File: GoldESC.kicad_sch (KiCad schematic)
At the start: 42 parts, among them J30 CanOut, J4 GND, J5 DB15_Female_HighDensity, J81 Conn_02x07_Counter_Clockwise, U2 FD8288T (DRV8300), U30 MCP2551-I-SN, U31 CPDT-12V, U80 STM32F103CBTx, U81 ABM3B-8.000MHZ

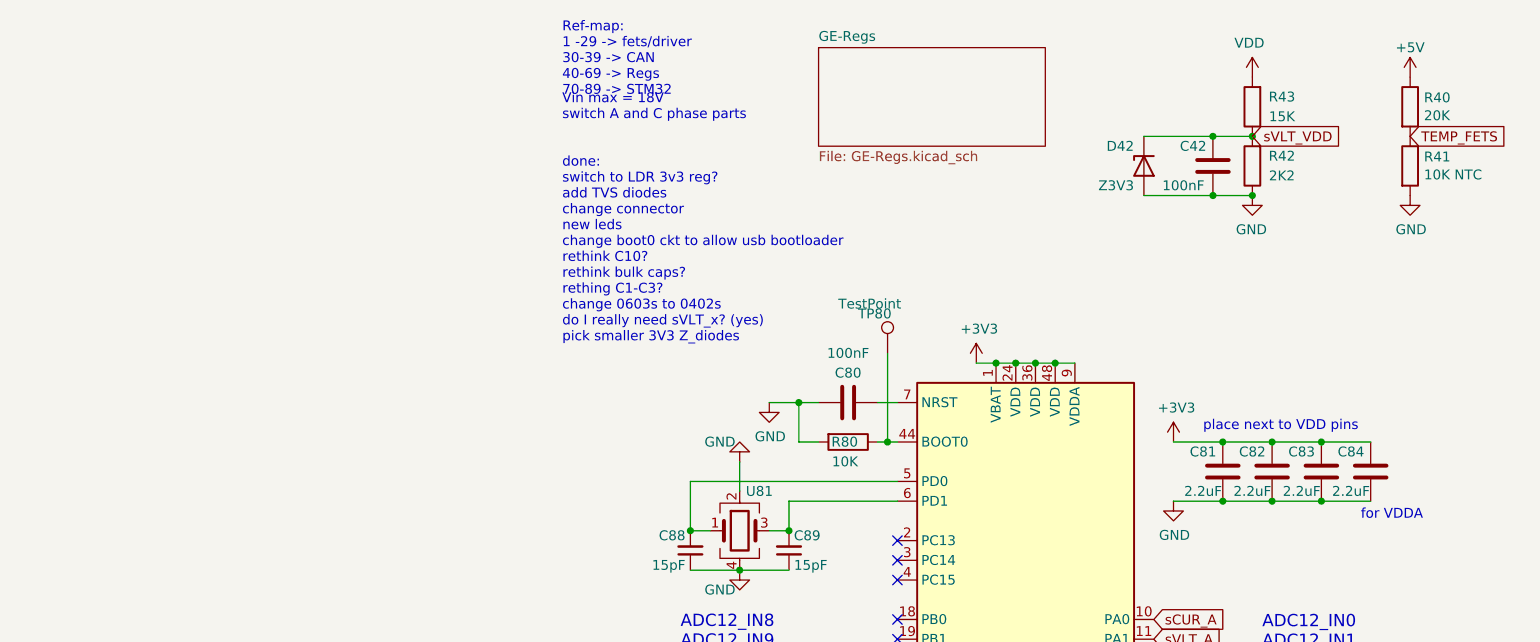
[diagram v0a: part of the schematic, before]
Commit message: updated gitignore
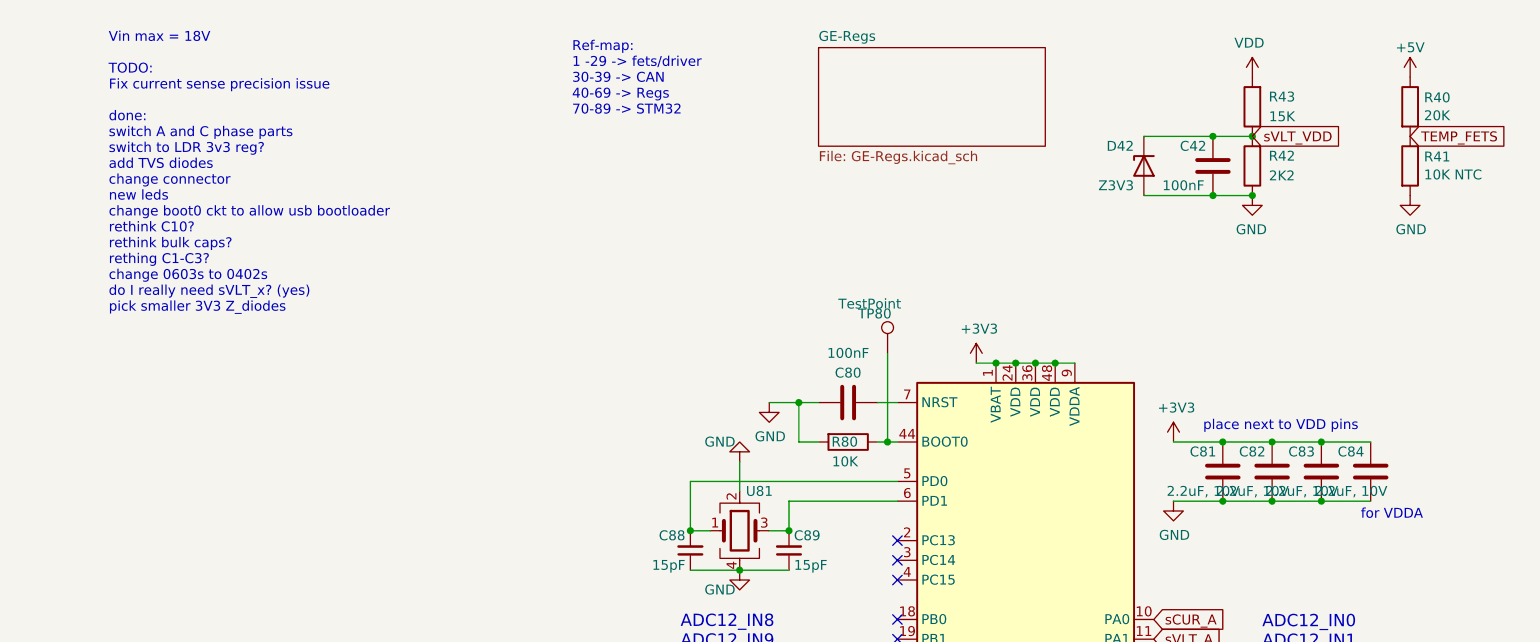
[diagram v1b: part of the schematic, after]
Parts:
- C81, C82, C83, C84: value 2.2uF -> 2.2uF, 10V; LCSC C12530 -> C77002
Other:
- note added: "Vin max = 18V TODO: Fix current sense precision issue done: switch A and C phase parts switch to LDR 3v3 reg? add TVS diodes change connector new leds change boot0 ckt to allow usb bootloader rethink C10? rethink bulk caps? rething C1-C3? change 0603s to 0402s do I really need sVLT_x? (yes) pick smaller 3V3 Z_diodes"
- note removed: "Vin max = 18V switch A and C phase parts done: switch to LDR 3v3 reg? add TVS diodes change connector new leds change boot0 ckt to allow usb bootloader rethink C10? rethink bulk caps? rething C1-C3? change 0603s to 0402s do I really need sVLT_x? (yes) pick smaller 3V3 Z_diodes"
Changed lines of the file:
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@@
     (stroke (width 0) (type default) (color 0 0 0 0))
   )
-  (text "Vin max = 18V\nswitch A and C phase parts\n\n\ndone:\nswitch to LDR 3v3 reg?\nadd TVS diodes\nchange connector\nnew leds\nchange boot0 ckt to allow usb bootloader\nrethink C10?\nrethink bulk caps?\nrething C1-C3?\nchange 0603s to 0402s\ndo I really need sVLT_x? (yes)\npick smaller 3V3 Z_diodes"
-    (at 13.97 55.88 0)
+  (text "Vin max = 18V\n\nTODO:\nFix current sense precision issue\n\ndone:\nswitch A and C phase parts\nswitch to LDR 3v3 reg?\nadd TVS diodes\nchange connector\nnew leds\nchange boot0 ckt to allow usb bootloader\nrethink C10?\nrethink bulk caps?\nrething C1-C3?\nchange 0603s to 0402s\ndo I really need sVLT_x? (yes)\npick smaller 3V3 Z_diodes"
+    (at -44.45 52.07 0)
     (effects (font (size 1.27 1.27)) (justify left bottom))
   )
@@
   )
   (text "Ref-map:\n1 -29 -> fets/driver\n30-39 -> CAN\n40-69 -> Regs\n70-89 -> STM32"
-    (at 13.97 24.13 0)
+    (at 15.24 26.67 0)
     (effects (font (size 1.27 1.27)) (justify left bottom))
   )
@@
     (in_bom yes) (on_board yes)
     (property "Reference" "C83" (id 0) (at 109.22 69.85 0))
-    (property "Value" "2.2uF" (id 1) (at 109.22 74.93 0))
+    (property "Value" "2.2uF, 10V" (id 1) (at 109.22 74.93 0))
     (property "Footprint" "Capacitor_SMD:C_0402_1005Metric" (id 2) (at 112.7252 76.2 0)
       (effects (font (size 1.27 1.27)) hide)
     )
-    (property "Datasheet" "https://lcsc.com/product-detail/Multilayer-Ceramic-Capacitors-MLCC---SMD-SMT_Samsung-Electro-Mechanics-Samsung-Electro-Mechanics-CL05A225MQ5NSNC_C12530.html" (id 3) (at 111.76 72.39 0)
-      (effects (font (size 1.27 1.27)) hide)
-    )
-    (property "LCSC" "C12530" (id 4) (at 111.76 72.39 0)
+    (property "Datasheet" "https://lcsc.com/product-detail/Multilayer-Ceramic-Capacitors-MLCC---SMD-SMT_Murata-Electronics-Murata-Electronics-GRM155R61A225KE95D_C77002.html" (id 3) (at 111.76 72.39 0)
+      (effects (font (size 1.27 1.27)) hide)
+    )
+    (property "LCSC" "C77002" (id 4) (at 111.76 72.39 0)
       (effects (font (size 1.27 1.27)) hide)
     )
@@
       (effects (font (size 1.27 1.27)) hide)
     )
-    (property "Datasheet" "https://lcsc.com/product-detail/Chip-Resistor-Surface-Mount_UNI-ROYAL-Uniroyal-Elec-0402WGF2201TCE_C25879.html" (id 3) (at 102.87 33.02 0)
+    (property "Datasheet" "" (id 3) (at 102.87 33.02 0)
       (effects (font (size 1.27 1.27)) hide)
     )
@@
     (in_bom yes) (on_board yes)
     (property "Reference" "C84" (id 0) (at 115.57 69.85 0))
-    (property "Value" "2.2uF" (id 1) (at 115.57 74.93 0))
+    (property "Value" "2.2uF, 10V" (id 1) (at 115.57 74.93 0))
     (property "Footprint" "Capacitor_SMD:C_0402_1005Metric" (id 2) (at 119.0752 76.2 0)
       (effects (font (size 1.27 1.27)) hide)
     )
-    (property "Datasheet" "https://lcsc.com/product-detail/Multilayer-Ceramic-Capacitors-MLCC---SMD-SMT_Samsung-Electro-Mechanics-Samsung-Electro-Mechanics-CL05A225MQ5NSNC_C12530.html" (id 3) (at 118.11 72.39 0)
-      (effects (font (size 1.27 1.27)) hide)
-    )
-    (property "LCSC" "C12530" (id 4) (at 118.11 72.39 0)
+    (property "Datasheet" "https://lcsc.com/product-detail/Multilayer-Ceramic-Capacitors-MLCC---SMD-SMT_Murata-Electronics-Murata-Electronics-GRM155R61A225KE95D_C77002.html" (id 3) (at 118.11 72.39 0)
+      (effects (font (size 1.27 1.27)) hide)
+    )
+    (property "LCSC" "C77002" (id 4) (at 118.11 72.39 0)
       (effects (font (size 1.27 1.27)) hide)
     )
@@
     (in_bom yes) (on_board yes)
     (property "Reference" "C81" (id 0) (at 96.52 69.85 0))
-    (property "Value" "2.2uF" (id 1) (at 96.52 74.93 0))
+    (property "Value" "2.2uF, 10V" (id 1) (at 96.52 74.93 0))
     (property "Footprint" "Capacitor_SMD:C_0402_1005Metric" (id 2) (at 100.0252 76.2 0)
       (effects (font (size 1.27 1.27)) hide)
     )
-    (property "Datasheet" "https://lcsc.com/product-detail/Multilayer-Ceramic-Capacitors-MLCC---SMD-SMT_Samsung-Electro-Mechanics-Samsung-Electro-Mechanics-CL05A225MQ5NSNC_C12530.html" (id 3) (at 99.06 72.39 0)
-      (effects (font (size 1.27 1.27)) hide)
-    )
-    (property "LCSC" "C12530" (id 4) (at 99.06 72.39 0)
+    (property "Datasheet" "https://lcsc.com/product-detail/Multilayer-Ceramic-Capacitors-MLCC---SMD-SMT_Murata-Electronics-Murata-Electronics-GRM155R61A225KE95D_C77002.html" (id 3) (at 99.06 72.39 0)
+      (effects (font (size 1.27 1.27)) hide)
+    )
+    (property "LCSC" "C77002" (id 4) (at 99.06 72.39 0)
       (effects (font (size 1.27 1.27)) hide)
     )
@@
     (in_bom yes) (on_board yes)
     (property "Reference" "C82" (id 0) (at 102.87 69.85 0))
-    (property "Value" "2.2uF" (id 1) (at 102.87 74.93 0))
+    (property "Value" "2.2uF, 10V" (id 1) (at 102.87 74.93 0))
     (property "Footprint" "Capacitor_SMD:C_0402_1005Metric" (id 2) (at 106.3752 76.2 0)
       (effects (font (size 1.27 1.27)) hide)
     )
-    (property "Datasheet" "https://lcsc.com/product-detail/Multilayer-Ceramic-Capacitors-MLCC---SMD-SMT_Samsung-Electro-Mechanics-Samsung-Electro-Mechanics-CL05A225MQ5NSNC_C12530.html" (id 3) (at 105.41 72.39 0)
-      (effects (font (size 1.27 1.27)) hide)
-    )
-    (property "LCSC" "C12530" (id 4) (at 105.41 72.39 0)
+    (property "Datasheet" "https://lcsc.com/product-detail/Multilayer-Ceramic-Capacitors-MLCC---SMD-SMT_Murata-Electronics-Murata-Electronics-GRM155R61A225KE95D_C77002.html" (id 3) (at 105.41 72.39 0)
+      (effects (font (size 1.27 1.27)) hide)
+    )
+    (property "LCSC" "C77002" (id 4) (at 105.41 72.39 0)
       (effects (font (size 1.27 1.27)) hide)
     )
@@
     )
     (path "/24f6087b-20cb-42de-be39-cbde0aafbae0/00000000-0000-0000-0000-000060470612"
-      (reference "C63") (unit 1) (value "22uF, 10V") (footprint "Capacitor_SMD:C_0402_1005Metric")
+      (reference "C63") (unit 1) (value "2.2uF, 10V") (footprint "Capacitor_SMD:C_0402_1005Metric")
     )
     (path "/a49bf60f-4742-49cb-96f1-9bf97eaa2ad2"
@@
     )
     (path "/c1ac3d87-a0ec-4da6-a2ca-9780ffb9e4de"
-      (reference "C81") (unit 1) (value "2.2uF") (footprint "Capacitor_SMD:C_0402_1005Metric")
+      (reference "C81") (unit 1) (value "2.2uF, 10V") (footprint "Capacitor_SMD:C_0402_1005Metric")
     )
     (path "/e40cc072-f36e-40cf-a546-5216a23725e6"
-      (reference "C82") (unit 1) (value "2.2uF") (footprint "Capacitor_SMD:C_0402_1005Metric")
+      (reference "C82") (unit 1) (value "2.2uF, 10V") (footprint "Capacitor_SMD:C_0402_1005Metric")
     )
     (path "/051ed6a4-68d3-43d0-8a51-e9364a9f81d4"
-      (reference "C83") (unit 1) (value "2.2uF") (footprint "Capacitor_SMD:C_0402_1005Metric")
+      (reference "C83") (unit 1) (value "2.2uF, 10V") (footprint "Capacitor_SMD:C_0402_1005Metric")
     )
     (path "/22c00ebc-a7bc-455e-aced-e13977e8fbae"
-      (reference "C84") (unit 1) (value "2.2uF") (footprint "Capacitor_SMD:C_0402_1005Metric")
+      (reference "C84") (unit 1) (value "2.2uF, 10V") (footprint "Capacitor_SMD:C_0402_1005Metric")
     )
     (path "/17587fbe-62d4-47c6-87d6-4f4bde1f7881"
